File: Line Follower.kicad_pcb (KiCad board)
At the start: 4 copper layers, 160 x 90 mm, 11 parts, among them J3 Conn_01x04, J4 Conn_01x06, J5 Conn_01x06, U1 Teensy4.1, U2 D42V55F5 5V Voltage Regulator, U3 TB67H420FTG Dual Motor Driver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, U4 Big MOSFET Slide Switch with 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, U5 QTRX-HD-15A

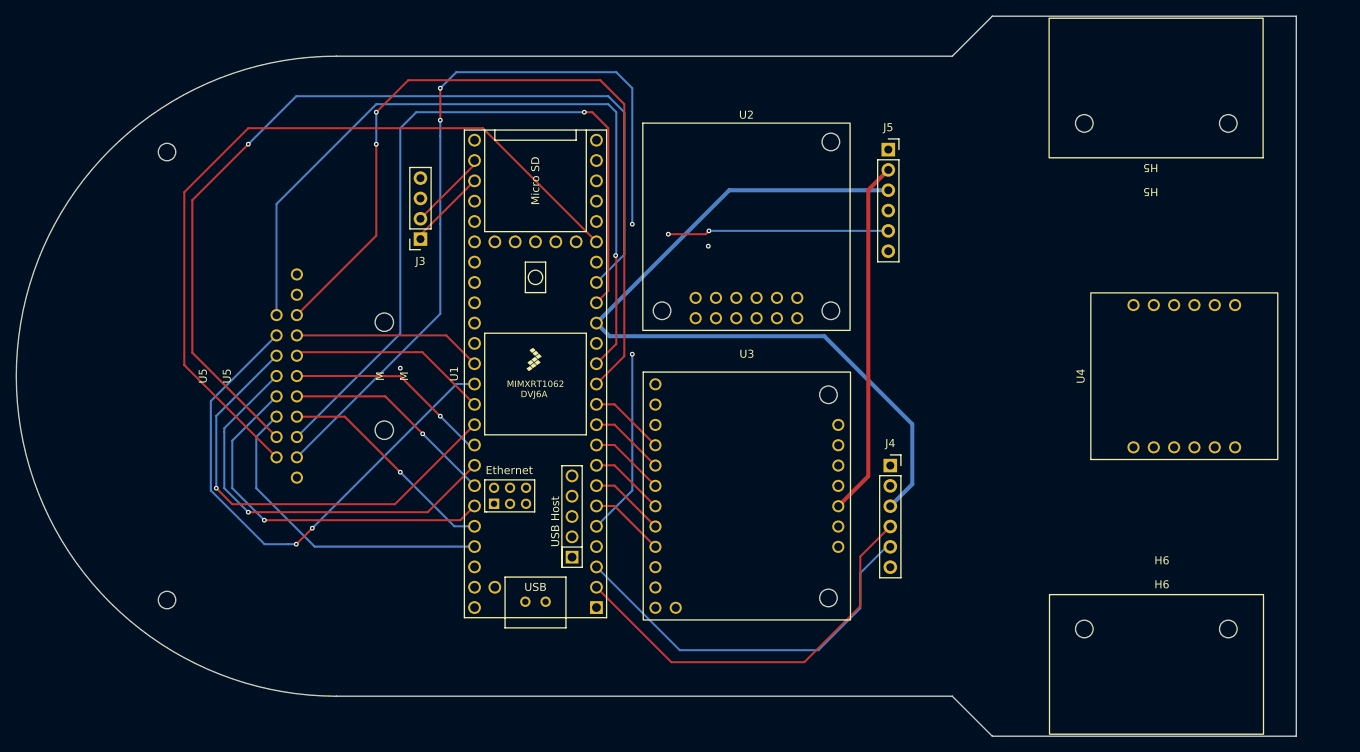
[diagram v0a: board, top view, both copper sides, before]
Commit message: Version1.0 QTRX-HD15A
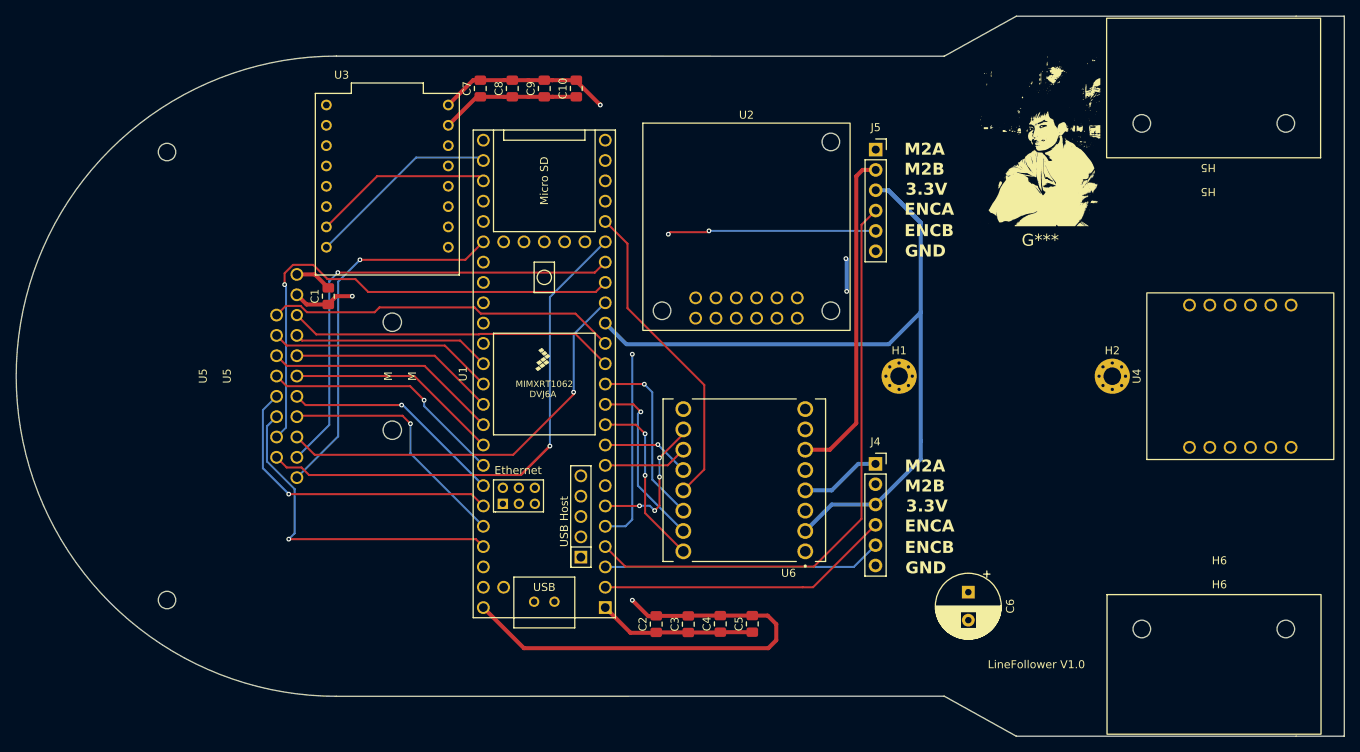
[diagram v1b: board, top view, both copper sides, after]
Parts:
- removed J3: Conn_01x04, Connector_PinSocket_2.54mm:PinSocket_1x04_P2.54mm_Vertical
- added C1: 0.1uF, Capacitor_SMD:C_0805_2012Metric_Pad1.18x1.45mm_HandSolder, F.Cu at (92.0, 82.0)
- added C10: 22uF, Capacitor_SMD:C_0805_2012Metric_Pad1.18x1.45mm_HandSolder, F.Cu at (123.0, 56.0)
- added C2: 0.1uF, Capacitor_SMD:C_0805_2012Metric_Pad1.18x1.45mm_HandSolder, F.Cu at (133.0, 123.0)
- added C3: 0.1uF, Capacitor_SMD:C_0805_2012Metric_Pad1.18x1.45mm_HandSolder, F.Cu at (137.0, 123.0)
- added C4: 0.1uF, Capacitor_SMD:C_0805_2012Metric_Pad1.18x1.45mm_HandSolder, F.Cu at (141.0, 123.0)
- added C5: 22uF, Capacitor_SMD:C_0805_2012Metric_Pad1.18x1.45mm_HandSolder, F.Cu at (145.0, 123.0)
- added C6: 470uF, Capacitor_THT:CP_Radial_D8.0mm_P3.50mm, F.Cu at (172.0, 119.0)
- added C7: 0.1uF, Capacitor_SMD:C_0805_2012Metric_Pad1.18x1.45mm_HandSolder, F.Cu at (111.0, 56.0)
- added C8: 0.1uF, Capacitor_SMD:C_0805_2012Metric_Pad1.18x1.45mm_HandSolder, F.Cu at (115.0, 56.0)
- added C9: 0.1uF, Capacitor_SMD:C_0805_2012Metric_Pad1.18x1.45mm_HandSolder, F.Cu at (119.0, 56.0)
- added G***: LOGO, logo:TestSymol, F.Cu at (181.0, 62.0)
- added H1: MountingHole_Pad, MountingHole:MountingHole_2.2mm_M2_Pad_Via, F.Cu at (163.3, 92.0)
- added H2: MountingHole_Pad, MountingHole:MountingHole_2.2mm_M2_Pad_Via, F.Cu at (190.0, 92.0)
- added U6: TB6612FNG BreakoutBoard, Pololu:MODULE_ROB-14450, F.Cu at (144.0, 105.0)
- U3: value TB67H420FTG Dual Motor Driver Carrier -> ESP32-C3_SUPERMINI_TH; footprint Pololu:TB67H420FTG Dual Motor Driver Carrier -> ESP32-C3_SUPERMINI_TH:MODULE_ESP32-C3_SUPERMINI_TH
- moved U3 63.1 mm to (99.4, 68.0)
- moved H5 7.19 mm to (202.7, 56.0)
- moved H6 7.19 mm to (202.7, 128.0)
- moved U4 7.00 mm to (217.4, 102.2)
- moved J4 1.86 mm to (160.4, 103.0)
- moved J5 1.57 mm to (160.4, 63.7)
- moved U1 1.10 mm to (119.0, 91.7)
- moved M 1.00 mm to (100.0, 92.0)
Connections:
- U1 pad 10: /M1INB -> /M1PWM
- U1 pad 11: /M1INA -> /M1INB
- U1 pad 12: /QTRXODD -> /M1INA
- U1 pad 13: /QTRXEVN -> /QTRXODD
- U1 pad 14: unconnected-(U1-12_MISO_MQSL_D12-Pad14) -> /QTRXEVN
- U1 pad 20: unconnected-(U1-28_RX7_D28-Pad20) -> /STBY
- U1 pad 26: /ESP8266 TX8 -> /ESP32 TX8
- U1 pad 27: /ESP8266 RX8 -> /ESP32 RX8
- U1 pad 7: /M2INB -> unconnected-(U1-5_IN2_D5-Pad7)
- U1 pad 8: /M2INA -> /M2INB
- U1 pad 9: /M1PWM -> /M2INA
- U3 pad 20: /M1A -> /ESP32 RX8
- U3 pad 4: /M1INA -> unconnected-(U3-GPIO4-Pad4)
- U3 pad 5: /M1INB -> unconnected-(U3-GPIO5-Pad5)
- U3 pad 6: /M1PWM -> unconnected-(U3-GPIO6-Pad6)
- U3 pad 7: /M2INA -> unconnected-(U3-GPIO7-Pad7)
- U3 pad 8: /M2INB -> unconnected-(U3-GPIO8-Pad8)
- U3 pad 9: /M2PWM -> unconnected-(U3-GPIO9-Pad9)
- U4 pad 10: GND -> unconnected-(U4-GND-Pad10)
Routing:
- net /QTRXODD: track 99.8 -> 41.1 mm, vias 2 -> 0
- net /QTRX12: track 116.9 -> 63.4 mm
- net /QTRXEVN: track 94.5 -> 44.0 mm, vias 1 -> 0
- net /QTRX13: track 102.8 -> 59.2 mm, vias 3 -> 1
- net GND: track 0.00 -> 42.6 mm
- net /QTRX11: track 94.0 -> 51.7 mm
- net /STBY: track 0.00 -> 39.8 mm
- net /QTRX2: track 66.8 -> 28.4 mm, vias 2 -> 0
- net +12V: track 96.8 -> 131.5 mm
- net /QTRX4: track 56.9 -> 29.4 mm, vias 1 -> 0
- net +5V: track 124.1 -> 149.8 mm, vias 0 -> 2
- net /ESP32 TX8: track 0.00 -> 24.4 mm
- net /QTRX14: track 98.6 -> 75.2 mm, vias 0 -> 1
- net /ESP32 RX8: track 0.00 -> 22.5 mm
- net /QTRX6: track 52.2 -> 30.9 mm
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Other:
- board size 160 x 90 mm -> 166 x 90 mm
- board text added: "3.3V"
- board text added: "ENCA"
- board text added: "ENCB"
- board text added: "GND"
- board text added: "LineFollower V1.0"
- board text added: "M2A"
- board text added: "M2B"
